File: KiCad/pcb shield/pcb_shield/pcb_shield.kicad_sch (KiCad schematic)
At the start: 25 parts, among them J1 , J10 Motor Conn L, J11 Motor Conn R, J12 Endstop X, J13 Endstop Y, J14 Barrel_Jack, J2 , J3 , J4 , J5 , J6 , J7 , J8 , J9 E_Magnet, Q1 TIP120, U1 BOB-09056, U2 BOB-09056, U3 BOB-09056, U4 BOB-09056

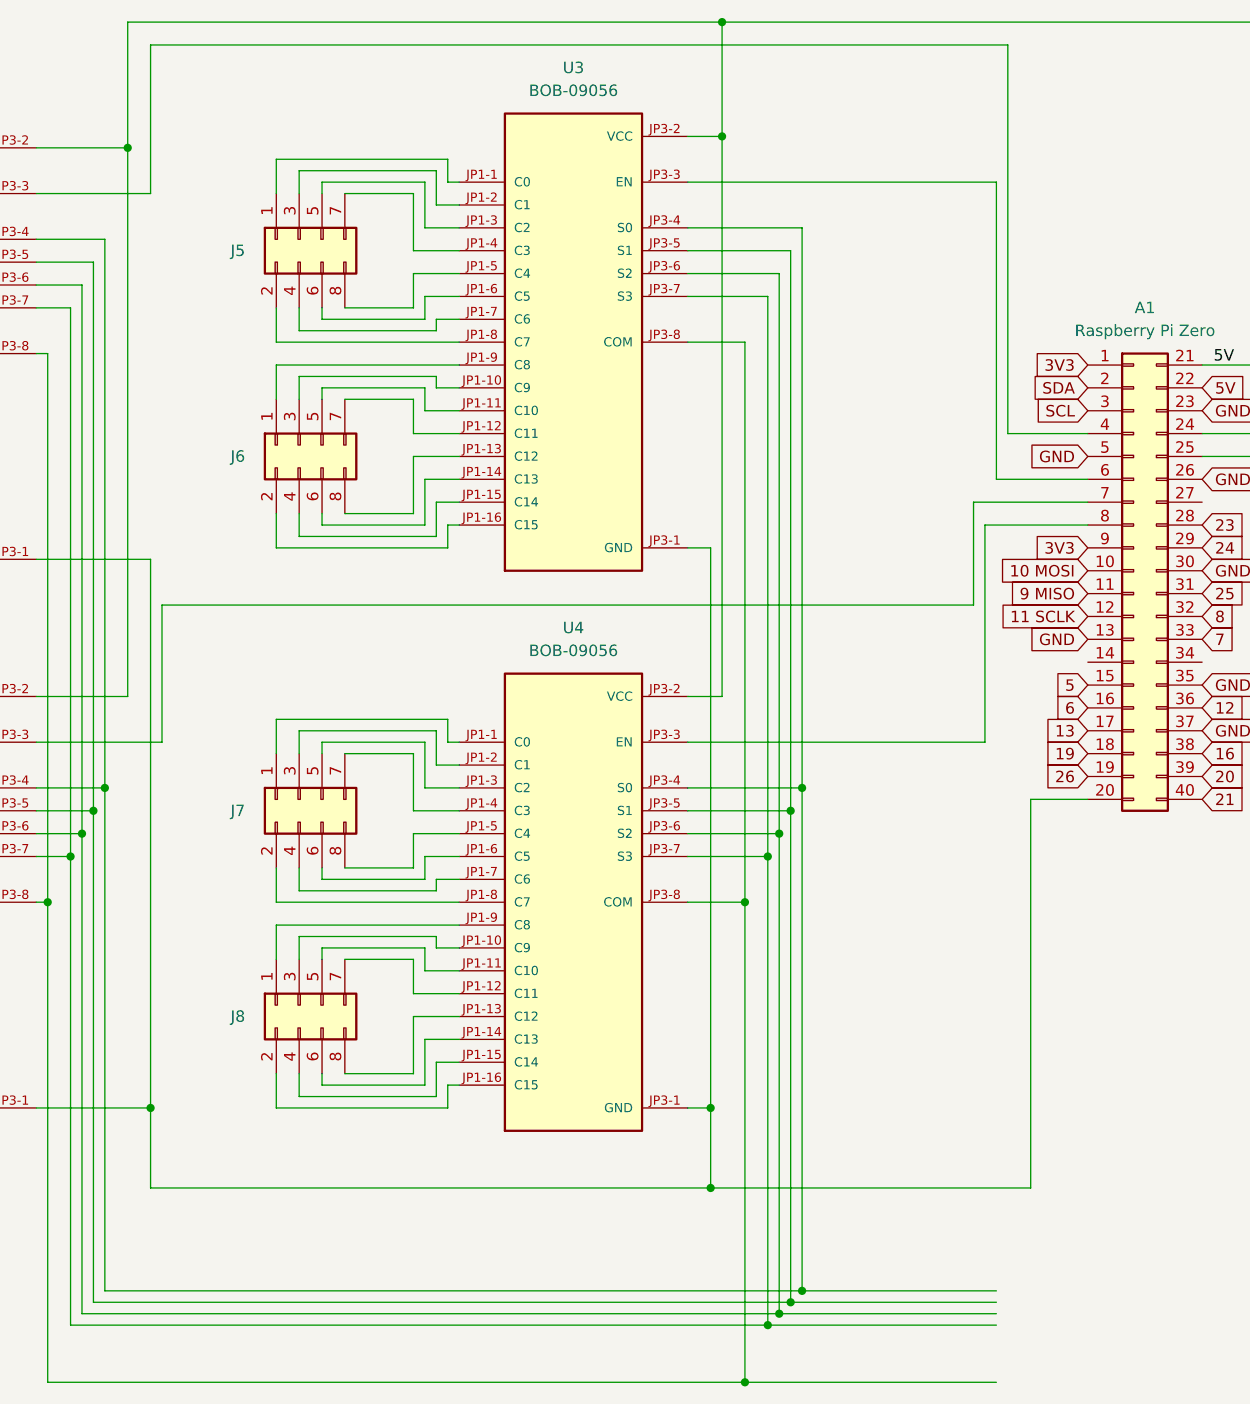
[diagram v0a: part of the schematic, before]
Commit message: almost finished pcb
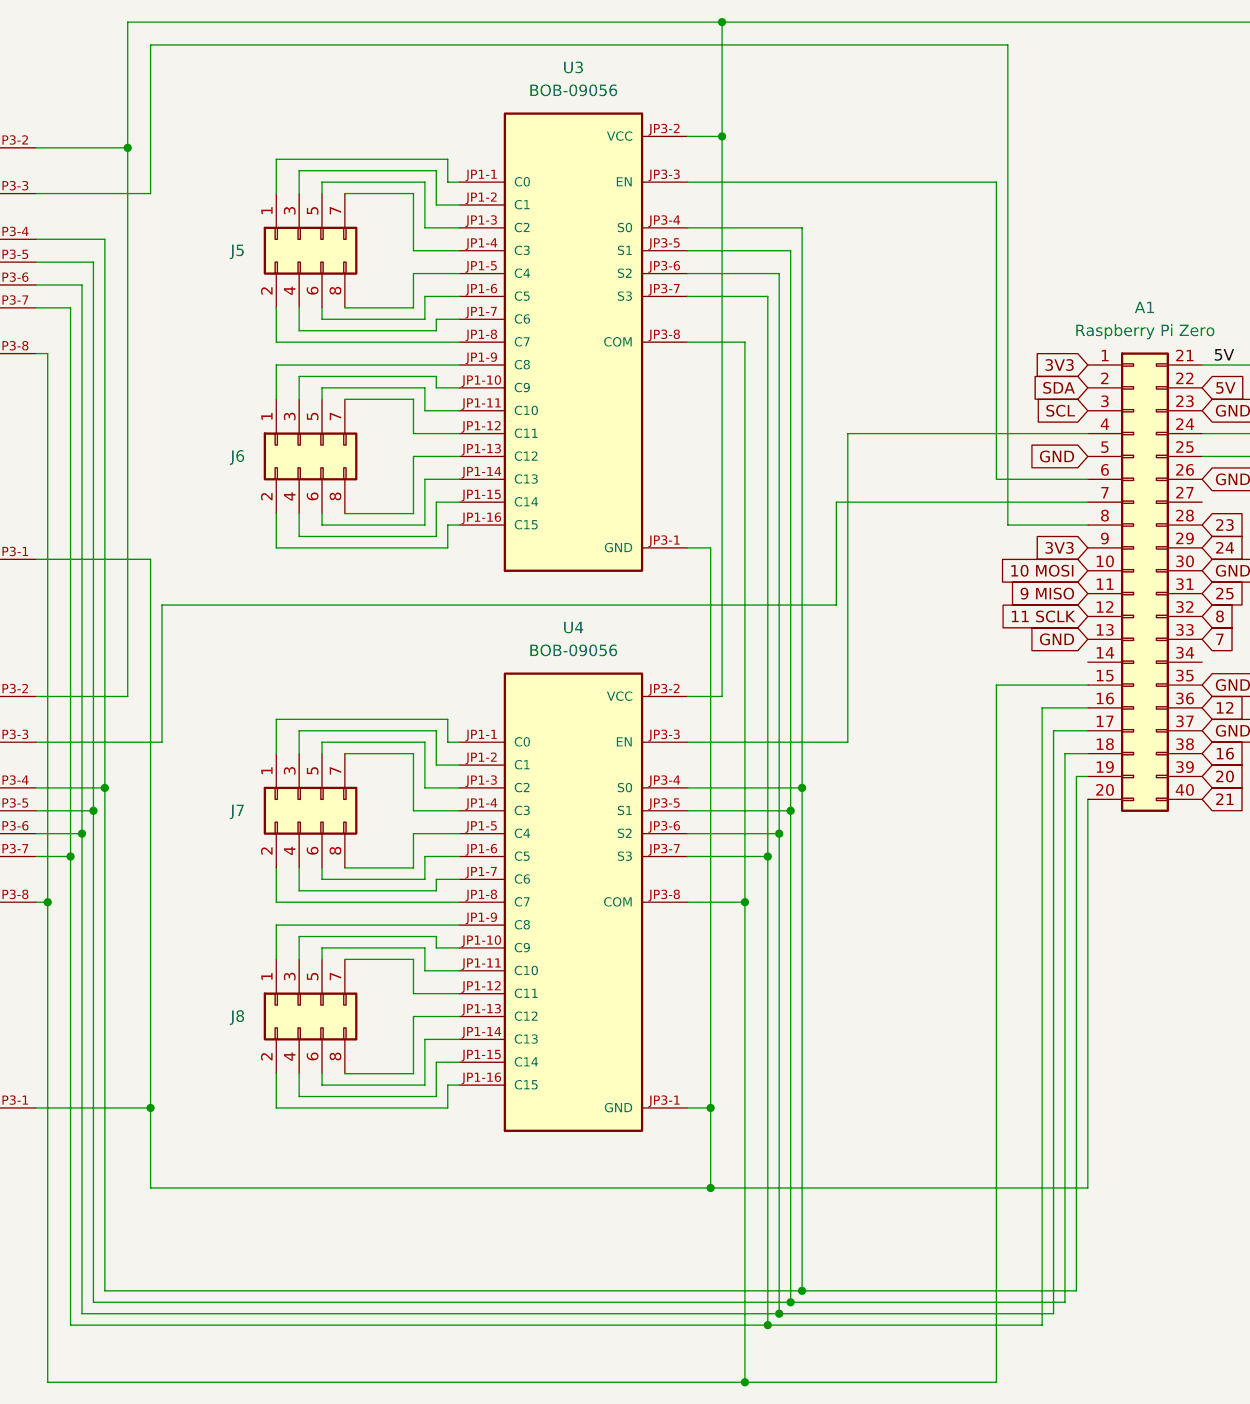
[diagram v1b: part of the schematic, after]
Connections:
- net 13 is gone; now on an unnamed net: A1.17 (Pin_17)
- net 19 is gone; now on an unnamed net: A1.18 (Pin_18)
- net 26 is gone; now on an unnamed net: A1.19 (Pin_19)
- net 5 is gone; now on an unnamed net: A1.15 (Pin_15)
- net 6 is gone; now on an unnamed net: A1.16 (Pin_16)
- net at U1.JP3-3 (EN): now also A1.8 (Pin_8); no longer A1.4 (Pin_4)
- net at U4.JP3-3 (EN): now also A1.4 (Pin_4); no longer A1.8 (Pin_8)
